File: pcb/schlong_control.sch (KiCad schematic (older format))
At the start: 28 parts, among them P1 Power Connector, P2 Data Connector, U1 74HC595, U2 OPTO-TRIAC, U3 OPTO-TRIAC, U4 OPTO-TRIAC, U5 OPTO-TRIAC, U6 OPTO-TRIAC

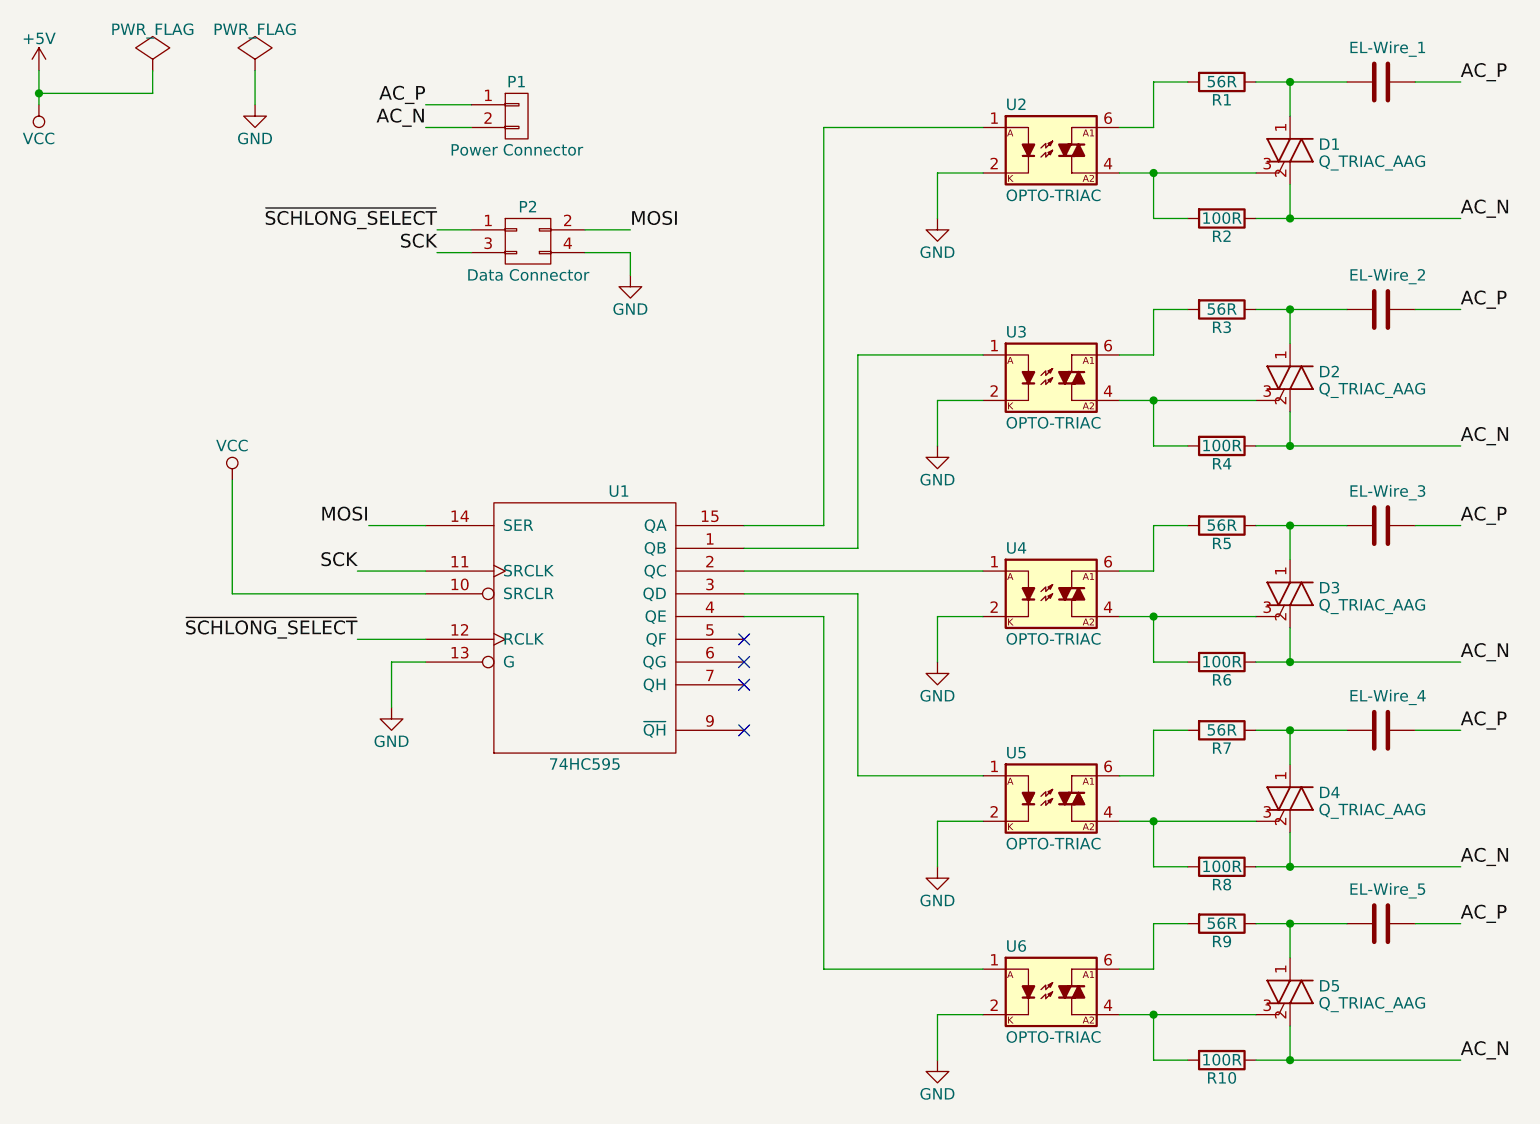
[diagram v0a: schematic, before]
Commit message: update circuit
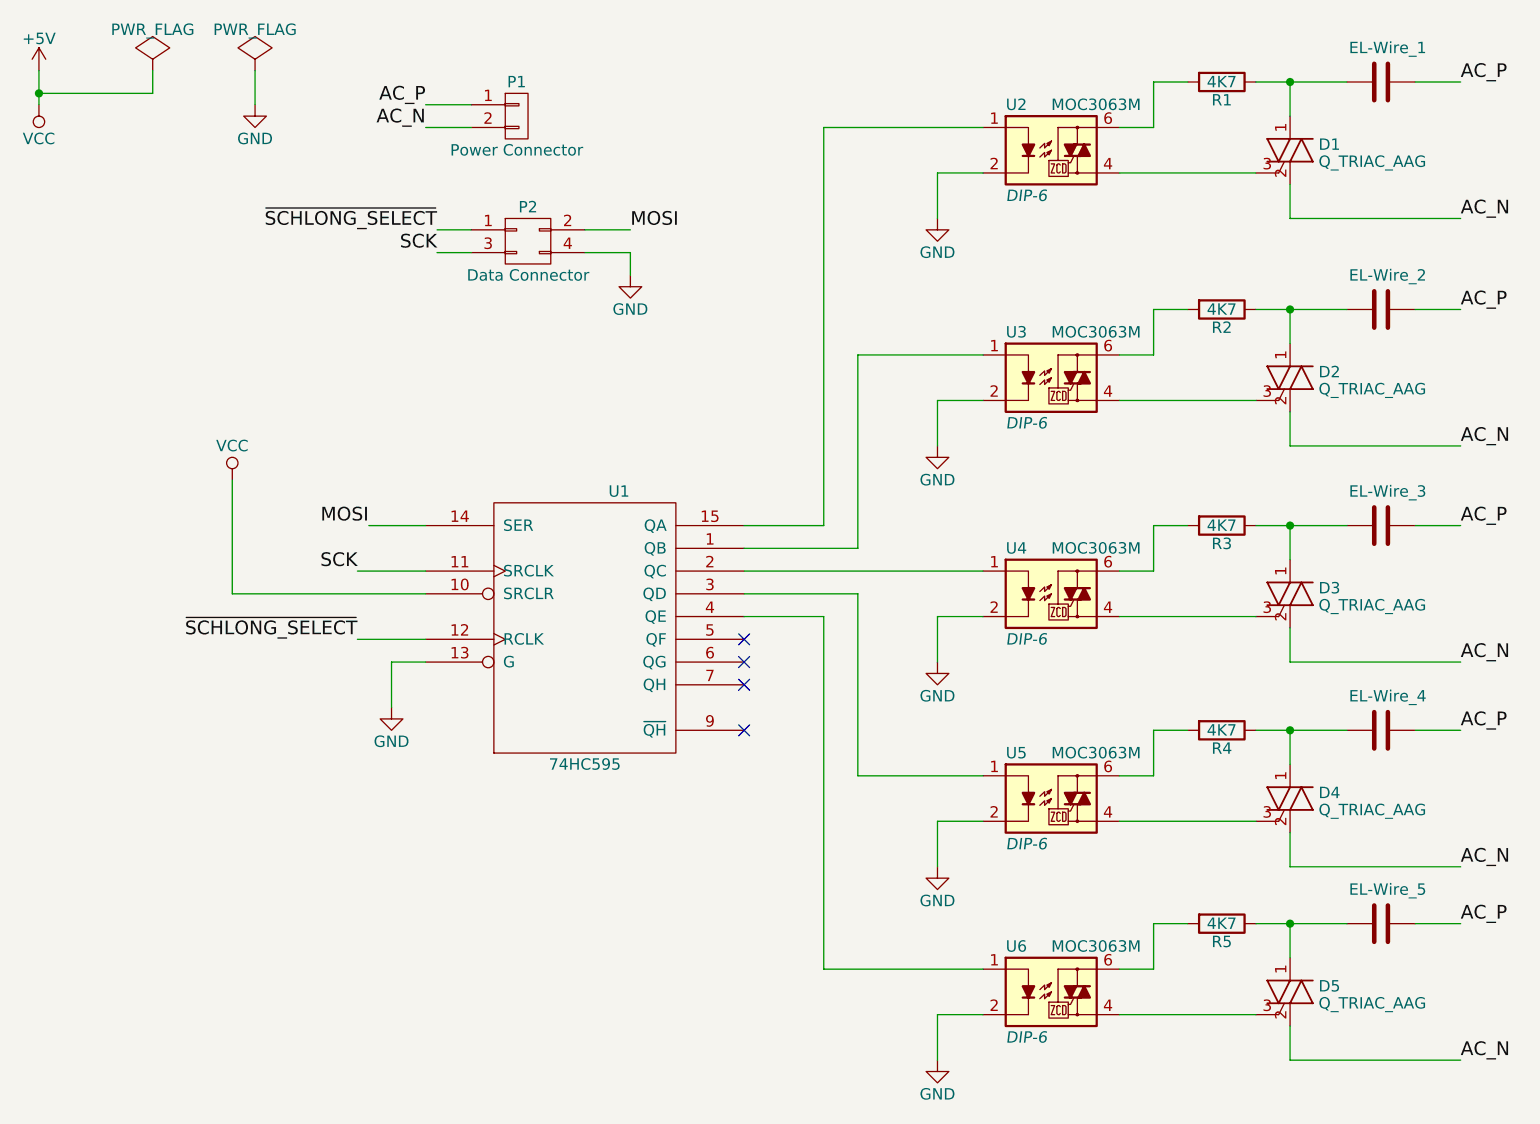
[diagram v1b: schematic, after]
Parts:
- removed R10, R2, R4, R6, R8: 100R, symbol R
- removed U2, U3, U4, U5, U6: OPTO-TRIAC, symbol OPTO-TRIAC
- added U2, U3, U4, U5, U6: MOC3063M, DIP-6, symbol MOC3063M
- R1: value 56R -> 4K7
- R2: renamed from R3; value 56R -> 4K7
- R3: renamed from R5; value 56R -> 4K7
- R4: renamed from R7; value 56R -> 4K7
- R5: renamed from R9; value 56R -> 4K7
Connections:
- net GND: now also U2.2, U3.2, U4.2, U5.2, U6.2
- net at U1.1 (QB): now also U3.1
- net at U1.15 (QA): now also U2.1
- net at U1.2 (QC): now also U4.1
- net at U1.3 (QD): now also U5.1
- net at U1.4 (QE): now also U6.1
- net at D1.3 (G): now also U2.4
- net at R1.2: now also U2.6
- net at D2.3 (G): now also U3.4
- net at R2.2: now also U3.6
- net at D3.3 (G): now also U4.4
- net at R3.2: now also U4.6
- net at D4.3 (G): now also U5.4
- net at R4.2: now also U5.6
- net at D5.3 (G): now also U6.4
- net at R5.2: now also U6.6
